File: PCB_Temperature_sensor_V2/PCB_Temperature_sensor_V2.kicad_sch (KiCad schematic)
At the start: 13 parts, among them J1 Conn_01x04_Pin, J2 Conn_01x02_Pin, J3 Conn_01x02_Pin, U2 LM358, U3 LM358

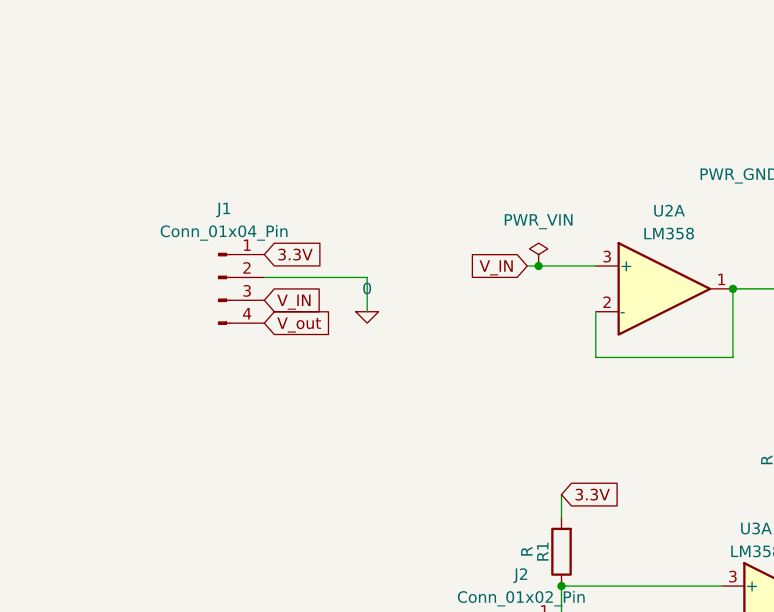
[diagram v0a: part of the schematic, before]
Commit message: V3
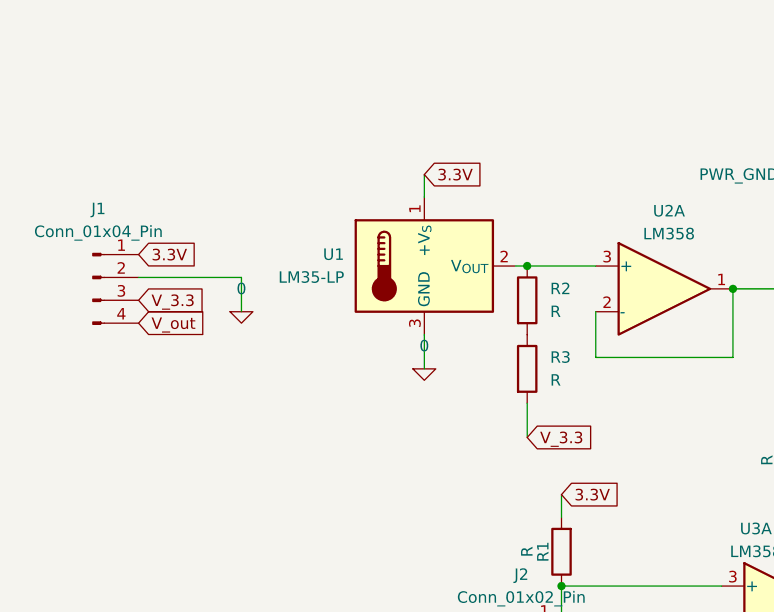
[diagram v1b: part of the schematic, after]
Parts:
- added R2, R3: R, Resistor_THT:R_Axial_DIN0207_L6.3mm_D2.5mm_P7.62mm_Horizontal, symbol Device:R
- added U1: LM35-LP, Package_TO_SOT_THT:TO-92_Inline, symbol Sensor_Temperature:LM35-LP
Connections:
- net 0: now also U1.3 (GND)
- net 3.3V: now also U1.1 (+V_{S})
- net V_IN: no longer names the net of U2.3 (+)
- net V_IN: now also R2.1, U1.2 (V_{OUT}); no longer J1.3 (Pin_3)
- new net: R2.2, R3.1
- new net V_3.3: J1.3 (Pin_3), R3.2
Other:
- moved on the sheet: J1
